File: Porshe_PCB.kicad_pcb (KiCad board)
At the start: 2 copper layers, 56.6 x 66.5 mm, 36 parts, among them J12 Conn_01x01_Pin, J14 Conn_02x20_Odd_Even, J16 Conn_02x20_Odd_Even, J2 SM04B-SRSS-TB_LF__SN_, J3 Conn_02x02_Odd_Even, J4 S2B-PH-SM4-TB_LF__SN_, J5 Screw_Terminal_01x03, J6 Conn_01x01_Pin, J7 Conn_01x01_Pin, J8 Conn_01x01_Pin, J9 Conn_02x04_Odd_Even, Q1 DMG2305UX-7, U1 DS3231SN, U2 AHT20

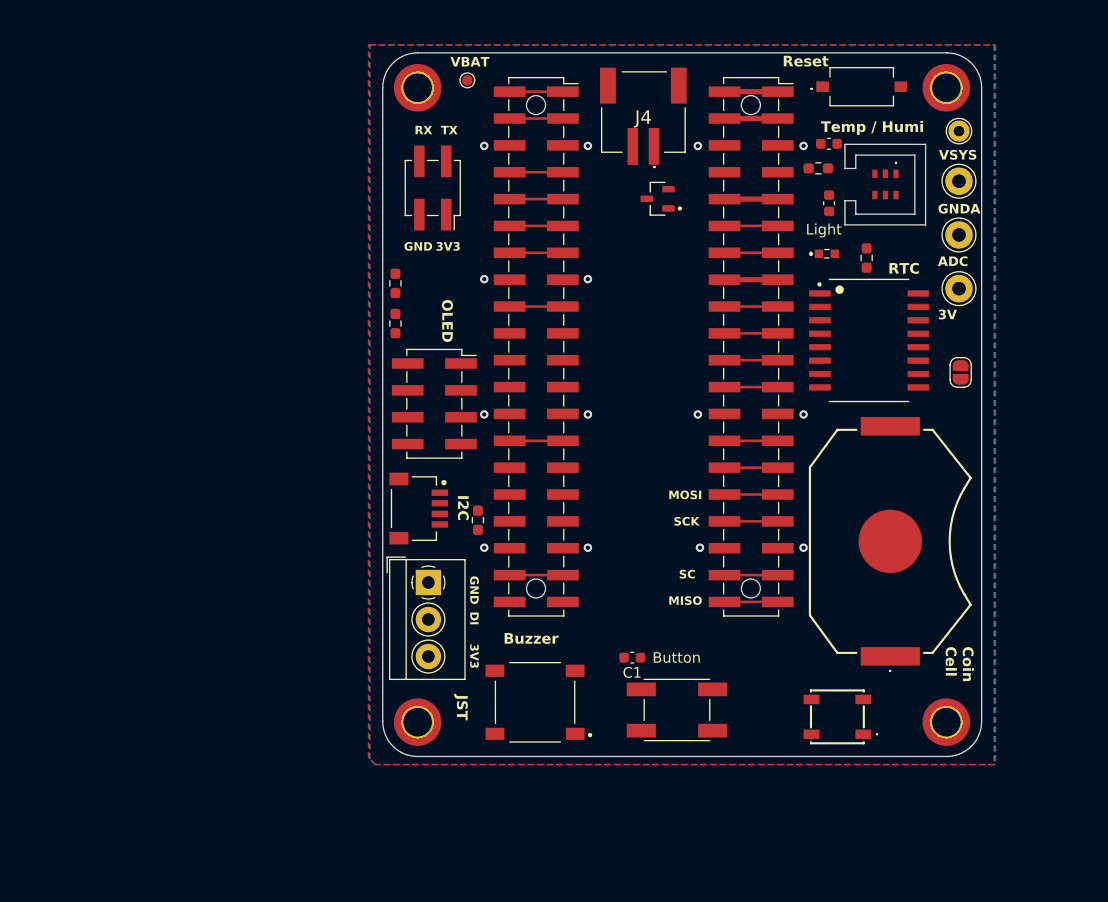
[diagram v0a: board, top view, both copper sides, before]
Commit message: 회로도 완성
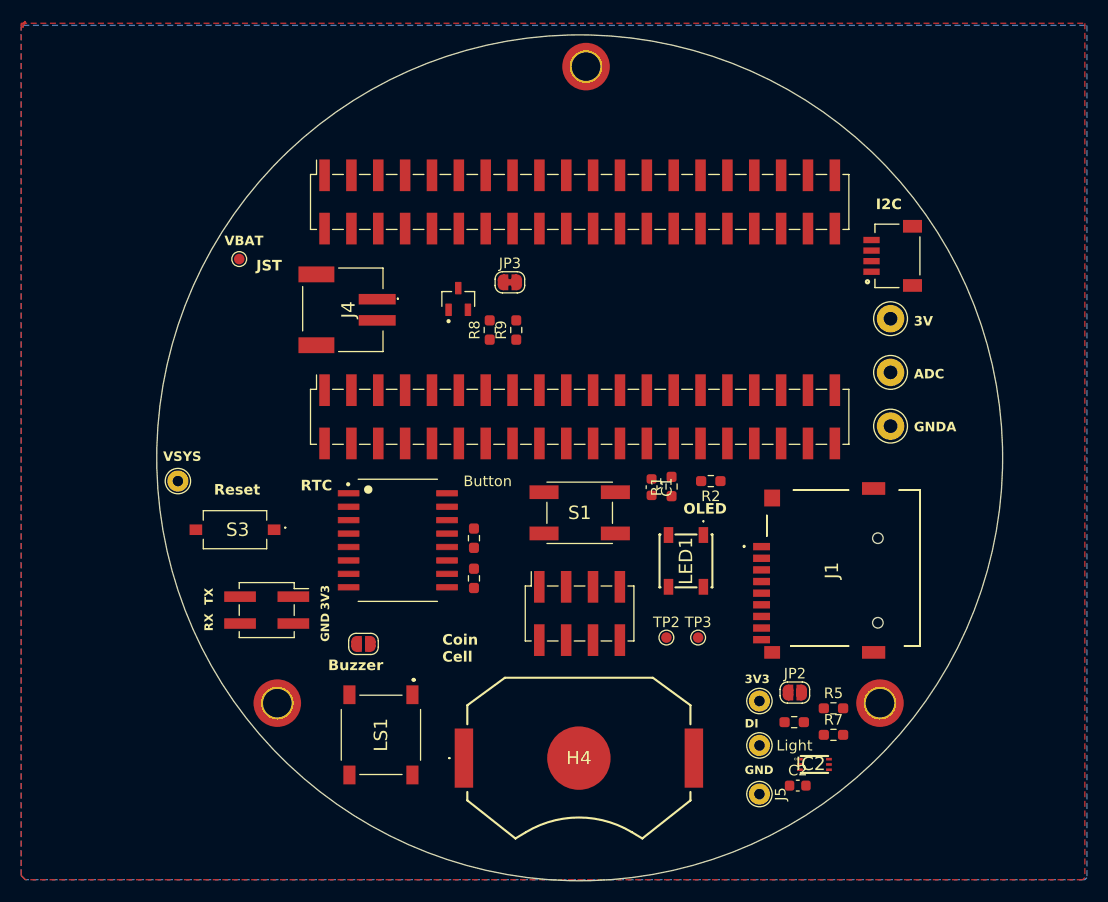
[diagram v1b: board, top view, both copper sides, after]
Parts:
- removed C5: 10uF/10V(10%), Capacitor_SMD:C_0603_1608Metric
- removed C6: 0.1uF/10V(10%), Capacitor_SMD:C_0603_1608Metric
- removed H5: MountingHole_Pad, MountingHole:MountingHole_2.7mm_M2.5_ISO7380_Pad_TopOnly
- removed U2: AHT20, AHT20:AHT20
- added C2: 1uF/50V(10%), Capacitor_SMD:C_0603_1608Metric, F.Cu at (153.2, 129.5)
- added IC2: BH1750FVI-TR, BH1750:WSOF6, F.Cu at (154.8, 127.5)
- added J1: TF-115, TF-115:TF115, F.Cu at (156.5, 109.2)
- added J10: Conn_01x01_Pin, TestPoint:TestPoint_THTPad_D2.0mm_Drill1.0mm, F.Cu at (149.6, 121.5)
- added J11: Conn_01x01_Pin, TestPoint:TestPoint_THTPad_D2.0mm_Drill1.0mm, F.Cu at (149.6, 125.7)
- added JP2: Jumper_2_Open, Jumper:SolderJumper-2_P1.3mm_Open_RoundedPad1.0x1.5mm, F.Cu at (153.0, 120.7)
- added JP3: Jumper_2_Bridged, Jumper:SolderJumper-2_P1.3mm_Bridged_RoundedPad1.0x1.5mm, F.Cu at (126.0, 81.9)
- added R1: 4.7k, Resistor_SMD:R_0603_1608Metric_Pad0.98x0.95mm_HandSolder, F.Cu at (141.3, 101.2)
- added R2: 4.7k, Resistor_SMD:R_0603_1608Metric_Pad0.98x0.95mm_HandSolder, F.Cu at (145.0, 100.7)
- added R5: 1k, Resistor_SMD:R_0603_1608Metric_Pad0.98x0.95mm_HandSolder, F.Cu at (156.6, 122.2)
- added TP2: TestPoint, TestPoint:TestPoint_Pad_D1.0mm, F.Cu at (140.8, 115.5)
- added TP3: TestPoint, TestPoint:TestPoint_Pad_D1.0mm, F.Cu at (143.8, 115.5)
- J5: value Screw_Terminal_01x03 -> Conn_01x01_Pin; footprint TerminalBlock_4Ucon:TerminalBlock_4Ucon_1x03_P3.50mm_Horizontal -> TestPoint:TestPoint_THTPad_D2.0mm_Drill1.0mm
- R7: value ALS-PT19-315C_L177_TR8 -> 10k; footprint ALS-PT19-315C:ALSPT19315CL177TR8 -> Resistor_SMD:R_0603_1608Metric_Pad0.98x0.95mm_HandSolder
- R8: value 10K(5%) -> 10k
- R9: value 220 -> 10k
- moved H2 86.0 mm to (104.0, 121.7)
- moved J12 81.0 mm to (94.6, 100.7)
- moved S3 72.6 mm to (100.0, 105.3), turned to 180 degrees
- moved JP1 62.0 mm to (112.2, 116.1), turned to 180 degrees
- moved U1 48.4 mm to (115.4, 106.3)
- moved J2 47.3 mm to (160.2, 79.4), turned to 90 degrees
- moved R7 45.5 mm to (156.6, 124.7)
- moved H3 43.8 mm to (161.0, 121.7)
- moved J3 42.9 mm to (103.0, 112.9), turned to 0 degrees
- moved J5 37.2 mm to (149.6, 130.3)
- moved R8 36.3 mm to (124.1, 86.4), turned to 90 degrees
- moved H4 35.9 mm to (132.6, 126.9), turned to 0 degrees
- moved P1 35.9 mm to (132.6, 126.9)
- moved R6 35.5 mm to (152.9, 123.5), turned to 180 degrees
- moved J4 34.0 mm to (110.2, 84.5), turned to 90 degrees
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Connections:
- net /GP10 renamed /SPI1_SCK
- net /GP12 renamed /Light_RST
- net /SPI0_SCK renamed Net-(J14-Pin_33)
- J14 pad 17: /Light -> /BAT_DIV
- J14 pad 18: /Light -> /BAT_DIV
- J14 pad 31: /SPI0_MOSI -> Net-(J14-Pin_31)
- J14 pad 32: /SPI0_MOSI -> Net-(J14-Pin_31)
- J14 pad 37: /SPI_SC -> Net-(J14-Pin_37)
- J14 pad 38: /SPI_SC -> Net-(J14-Pin_37)
- J14 pad 39: /SPI0_MISO -> Net-(J14-Pin_39)
- J14 pad 40: /SPI0_MISO -> Net-(J14-Pin_39)
- J14 pad 7: unconnected-(J14-Pin_7-Pad7) -> Net-(J14-Pin_7)
- J14 pad 8: unconnected-(J14-Pin_8-Pad8) -> Net-(J14-Pin_7)
- J16 pad 21: unconnected-(J16-Pin_21-Pad21) -> /SPI0_MISO
- J16 pad 22: unconnected-(J16-Pin_22-Pad22) -> /SPI0_MISO
- J16 pad 23: /LED -> /SPI_SC
- J16 pad 24: /LED -> /SPI_SC
- J16 pad 29: /GP11 -> /SPI0_MOSI
- J16 pad 30: /GP11 -> /SPI0_MOSI
- J16 pad 33: /GP13 -> /LED
- J16 pad 34: /GP13 -> /LED
- J5 pad 1: GND -> /3V3
- R7 pad 1: /3V3 -> GND
- R7 pad 2: /Light -> Net-(IC2-ADDR)
- R8 pad 1: GNDA -> Net-(JP3-A)
- R8 pad 2: /Light -> /VBAT(+)
- R9 pad 1: Net-(U2-VDD) -> Net-(JP3-A)
- R9 pad 2: /3V3 -> /VBAT(+)
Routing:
- net Net-(J14-Pin_33): track 5.04 -> 0.00 mm
- net Net-(J14-Pin_29): track 5.04 -> 0.00 mm
- net Net-(J14-Pin_27): track 5.04 -> 0.00 mm
- net Net-(J14-Pin_19): track 5.04 -> 0.00 mm
- net Net-(J14-Pin_11): track 5.04 -> 0.00 mm
- net GNDA: track 5.04 -> 0.00 mm
- net /VSYS: track 5.04 -> 0.00 mm
- net /VBUS: track 5.04 -> 0.00 mm
- net /SPI_SC: track 5.04 -> 0.00 mm
- net /SPI0_MOSI: track 5.04 -> 0.00 mm
- net /SPI0_MISO: track 5.04 -> 0.00 mm
- net /RUN: track 5.04 -> 0.00 mm
- net /RTC_RST: track 5.04 -> 0.00 mm
- net /Light: track 5.04 -> 0.00 mm
- net /ADC2: track 5.04 -> 0.00 mm
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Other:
- board size 56.6 x 66.5 mm -> 80 x 80 mm
- board text removed: "MISO"
- board text removed: "MOSI"
- board text removed: "SC"
- board text removed: "SCK"
- board text removed: "Temp / Humi"
